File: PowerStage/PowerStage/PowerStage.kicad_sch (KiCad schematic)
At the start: 4 parts, among them J1 Conn_01x02, J2 Conn_01x02, J3 Conn_01x03, U1 IR2110

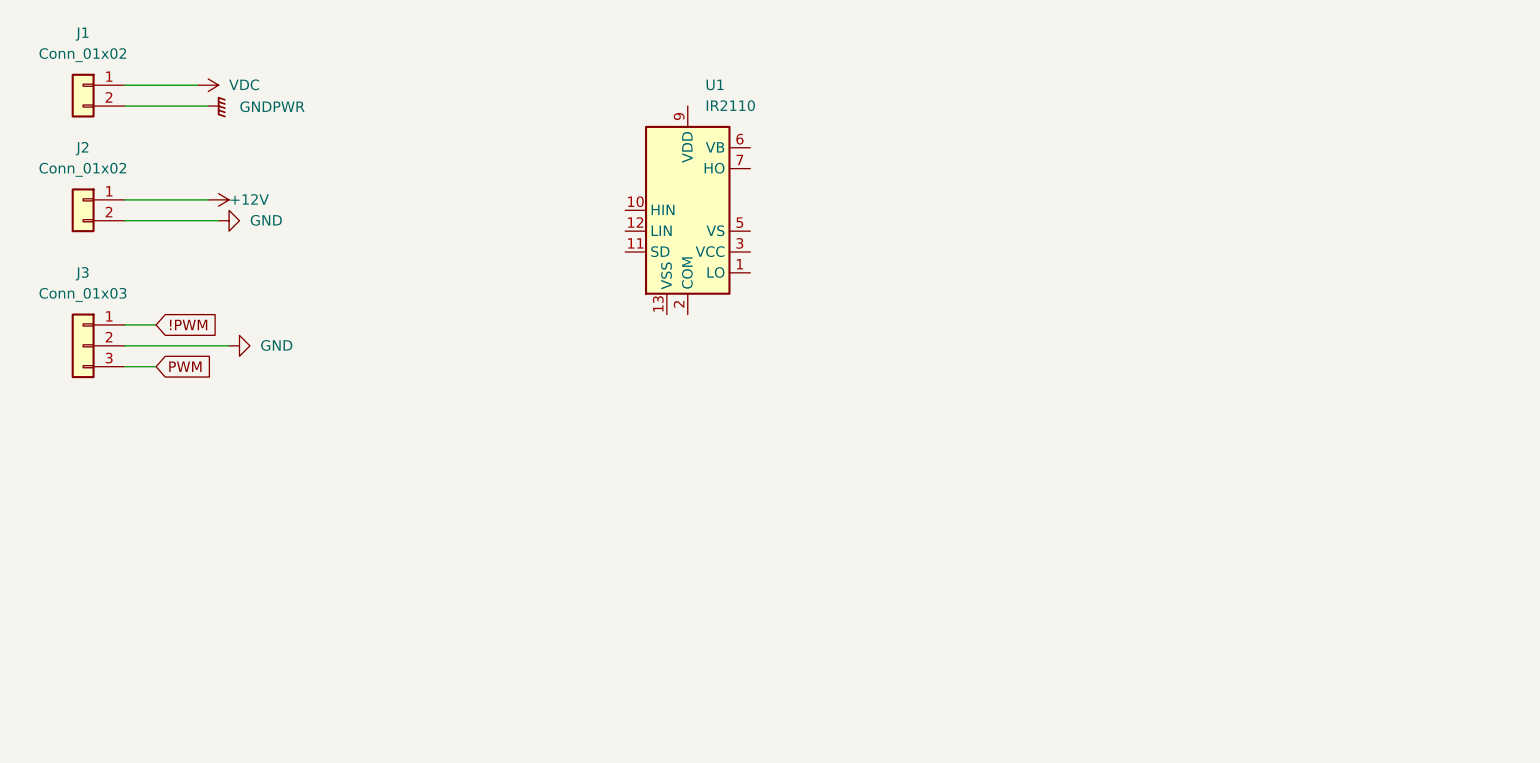
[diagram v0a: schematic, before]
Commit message: Finished power stage
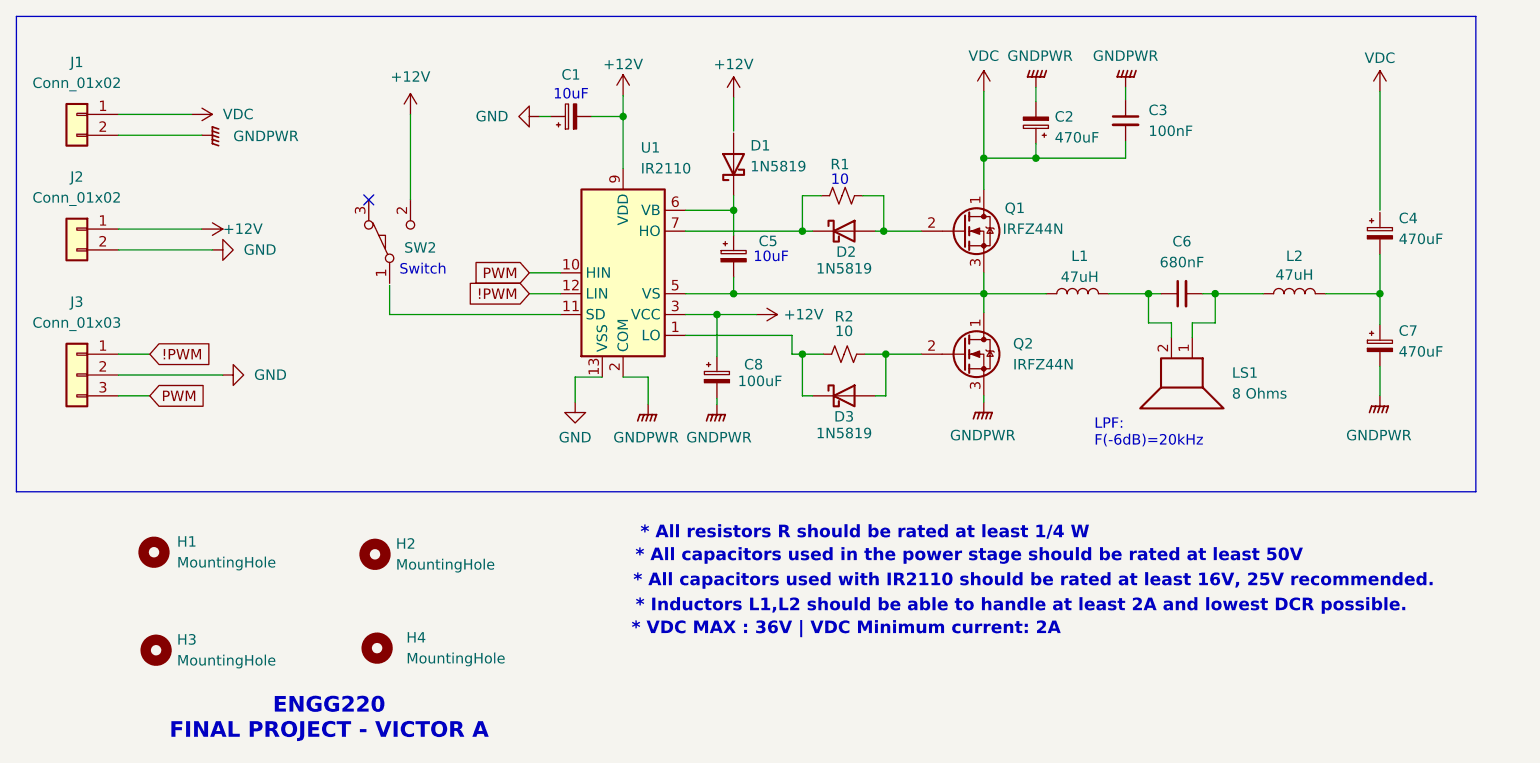
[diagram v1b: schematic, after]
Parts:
- added C1, C5: C_Polarized_Small, symbol Device:C_Polarized_Small
- added C2, C4, C7: 470uF, symbol Device:C_Polarized_Small
- added C3: 100nF, symbol Device:C_Small
- added C6: 680nF, symbol Device:C_Small
- added C8: 100uF, symbol Device:C_Polarized_Small
- added D1, D2, D3: 1N5819, Diode_THT:D_DO-41_SOD81_P10.16mm_Horizontal, symbol Diode:1N5819
- added H1, H2, H3, H4: MountingHole, symbol Mechanical:MountingHole
- added L1, L2: 47uH, symbol Device:L
- added LS1: 8 Ohms, symbol Device:Speaker
- added Q1, Q2: IRFZ44N, Package_DirectFET:DirectFET_MF, symbol Transistor_FET:IRF40DM229
- added R1: R_Small_US, symbol Device:R_Small_US
- added R2: 10, symbol Device:R_Small_US
- added SW2: SW_SPDT_XKB_DMx-xxxx-1, symbol Switch:SW_SPDT_XKB_DMx-xxxx-1
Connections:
- net !PWM: now also U1.12 (LIN)
- net +12V: now also U1.3 (VCC), U1.9 (VDD), C1.2, C8.1, SW2.2 (B)
- net GND: now also U1.13 (VSS), C1.1
- net GNDPWR: now also U1.2 (COM), C2.2, C3.1, C7.2, C8.2, Q2.3 (S)
- net PWM: now also U1.10 (HIN)
- net VDC: now also C2.1, C3.2, Q1.1 (D)
- net at U1.1 (LO): now also D3.1 (K), R2.1
- net at U1.5 (VS): now also C5.2, Q1.3 (S), Q2.1 (D)
- net at U1.6 (VB): now also C5.1, D1.1 (K)
- net at U1.7 (HO): now also D2.1 (K), R1.1
- new net: C4.2, C7.1, L2.2
- new net: C6.2, L2.1, LS1.1
- new net: C6.1, L1.2, LS1.2
- new net: D3.2 (A), Q2.2 (G), R2.2
- new net: D2.2 (A), Q1.2 (G), R1.2
- no-connect marks 0 -> 1
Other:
- note added: "* All capacitors used in the power stage should be rated at least 50V"
- note added: "* All capacitors used with IR2110 should be rated at least 16V, 25V recommended."
- note added: "* All resistors R should be rated at least 1/4 W"
- note added: "* Inductors L1,L2 should be able to handle at least 2A and lowest DCR possible."
- note added: "* VDC MAX : 36V | VDC Minimum current: 2A"
- note added: "10"
- note added: "10uF"
- note added: "ENGG220 FINAL PROJECT - VICTOR A"
- note added: "LPF: F(-6dB)=20kHz"
- note added: "Switch"
- title: (none) -> CLASS D POWER STAGE
- moved on the sheet: J1, J2, J3, U1
